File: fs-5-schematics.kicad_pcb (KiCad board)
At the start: 2 copper layers, 79 x 50 mm, 11 parts, among them U1 TPS54202DDC

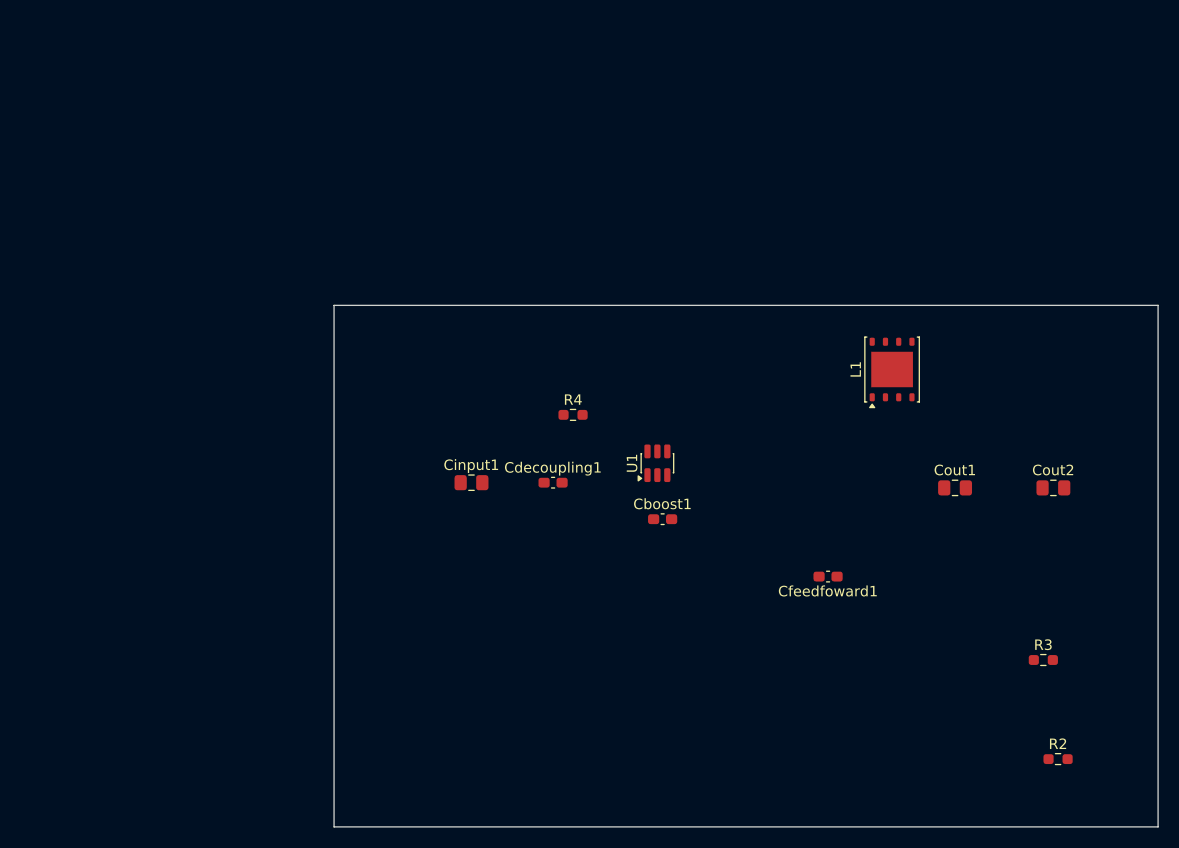
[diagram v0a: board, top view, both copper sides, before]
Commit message: PCb layouts complete?, need checked
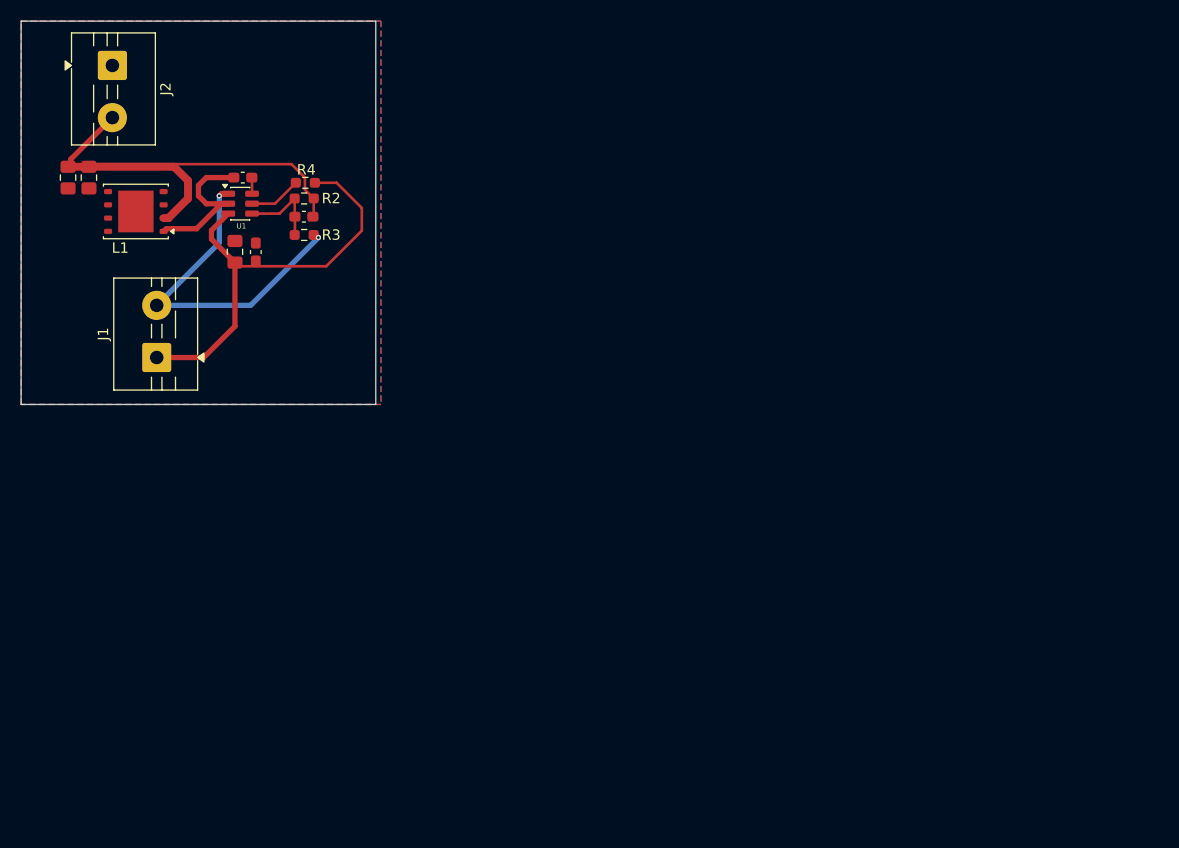
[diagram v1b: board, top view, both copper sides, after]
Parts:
- added J1: 12V, TerminalBlock:TerminalBlock_MaiXu_MX126-5.0-02P_1x02_P5.00mm, F.Cu at (82.0, 67.0)
- added J2: 5V, TerminalBlock:TerminalBlock_MaiXu_MX126-5.0-02P_1x02_P5.00mm, F.Cu at (77.8, 39.0)
- moved Cout2 99.0 mm to (73.5, 49.8), turned to -90 degrees
- moved R2 90.1 mm to (96.1, 51.8), turned to 180 degrees
- moved Cout1 88.2 mm to (75.5, 49.8), turned to -90 degrees
- moved R3 81.7 mm to (96.1, 55.2)
- moved L1 74.1 mm to (80.0, 53.0), turned to 180 degrees
- moved Cfeedfoward1 61.0 mm to (96.1, 53.5)
- moved Cboost1 51.9 mm to (90.2, 49.8), turned to 180 degrees
- moved U1 47.1 mm to (90.0, 52.2), turned to 0 degrees
- moved Cdecoupling1 36.1 mm to (91.5, 56.9), turned to 90 degrees
- moved R4 34.0 mm to (96.2, 50.2), turned to 180 degrees
- moved Cinput1 31.7 mm to (89.5, 56.9), turned to 90 degrees
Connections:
- Cfeedfoward1 pad 1: Net-(U1-FB) -> +5V
- Cfeedfoward1 pad 2: GND -> Net-(U1-FB)
- Cout1 pad 1: Net-(J2-Pin_2) -> +5V
- Cout2 pad 1: Net-(J2-Pin_2) -> +5V
- L1 pad 2: Net-(J2-Pin_2) -> +5V
- R2 pad 1: Net-(U1-FB) -> +5V
- R2 pad 2: GND -> Net-(U1-FB)
- R3 pad 1: Net-(J2-Pin_2) -> Net-(U1-FB)
- R3 pad 2: Net-(U1-FB) -> GND
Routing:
- net +5V: track 0.00 -> 48.8 mm
- net +12V: track 0.00 -> 42.5 mm
- net GND: track 0.00 -> 32.7 mm, vias 0 -> 2
- net Net-(U1-SW): track 0.00 -> 15.2 mm
- net Net-(U1-FB): track 0.00 -> 8.35 mm
- net Net-(U1-EN): track 0.00 -> 5.44 mm
- net Net-(U1-BOOT): track 0.00 -> 1.56 mm
- added copper zone on B.Cu, net GND
- added copper zone on F.Cu, net GND
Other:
- board size 79 x 50 mm -> 34 x 36.8 mm
